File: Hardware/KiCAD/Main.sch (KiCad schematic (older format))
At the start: 33 parts, among them J1 ICSP, J2 DB9, J3 DB9, J4 SPARE, U1 PIC18F25K80, U2 POXA1328-007, U3 RN4020, U4 S25FL127S_SOIC, U5 4000series-4052, U6 4000series-4052, U7 MCP795XX, U8 MAX3232_BJH, U9 MAX3232_BJH, Y1 12MHz, Y2 32.768Hz

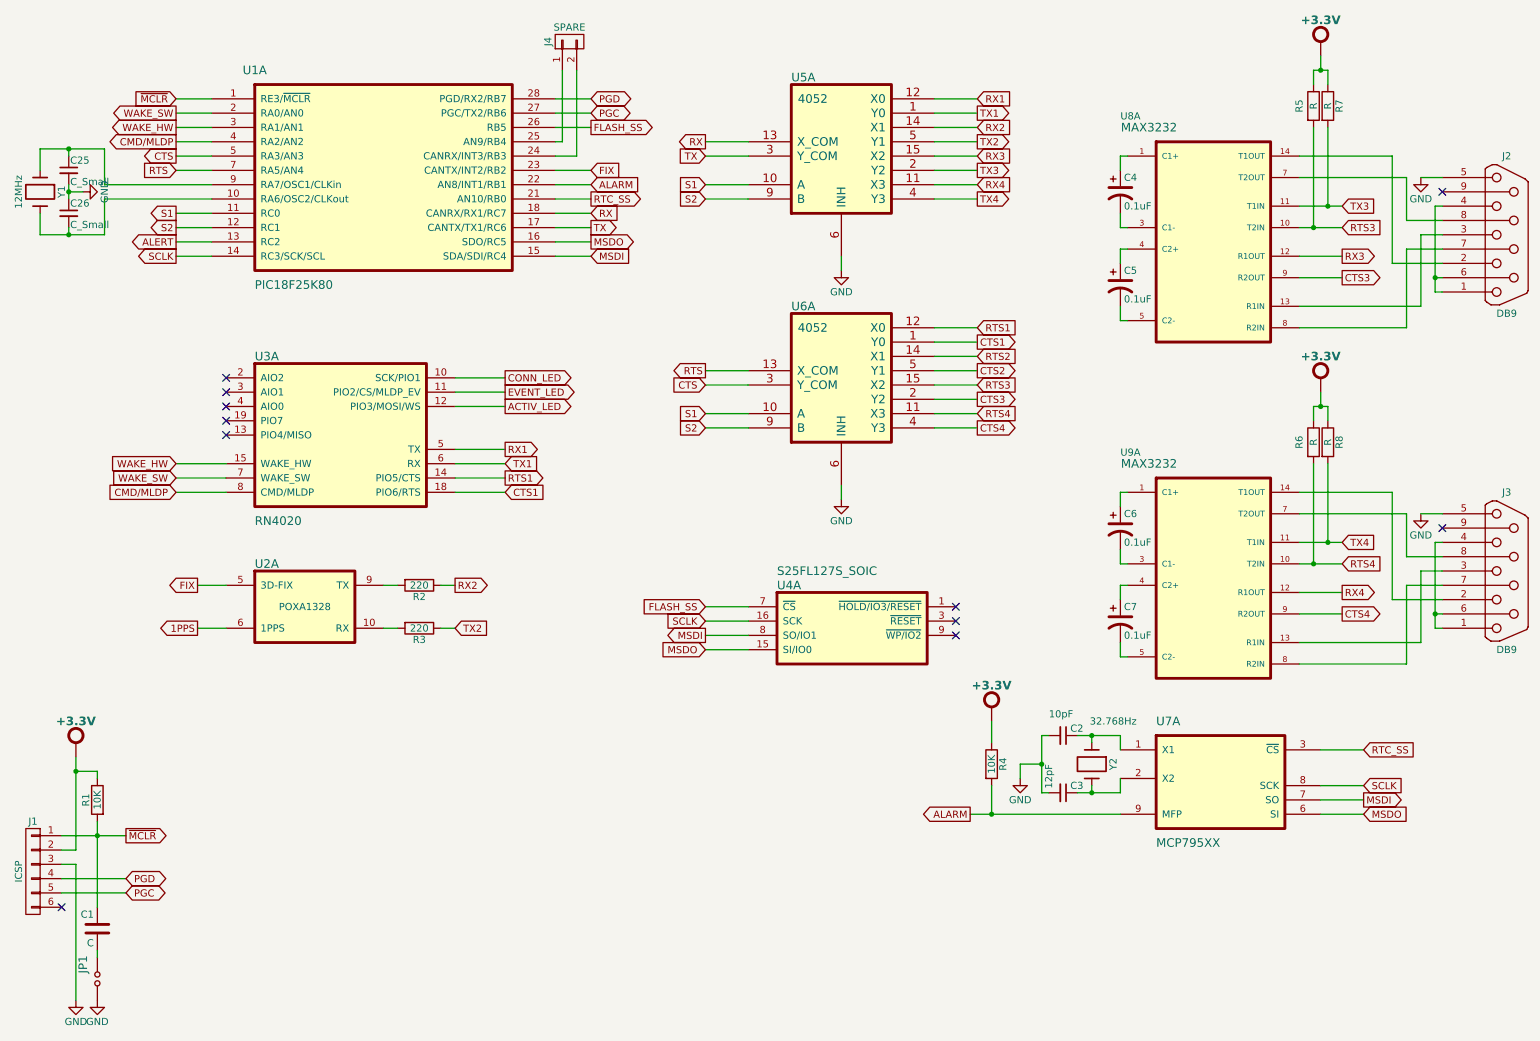
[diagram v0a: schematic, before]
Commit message: More work on PTWS schematic
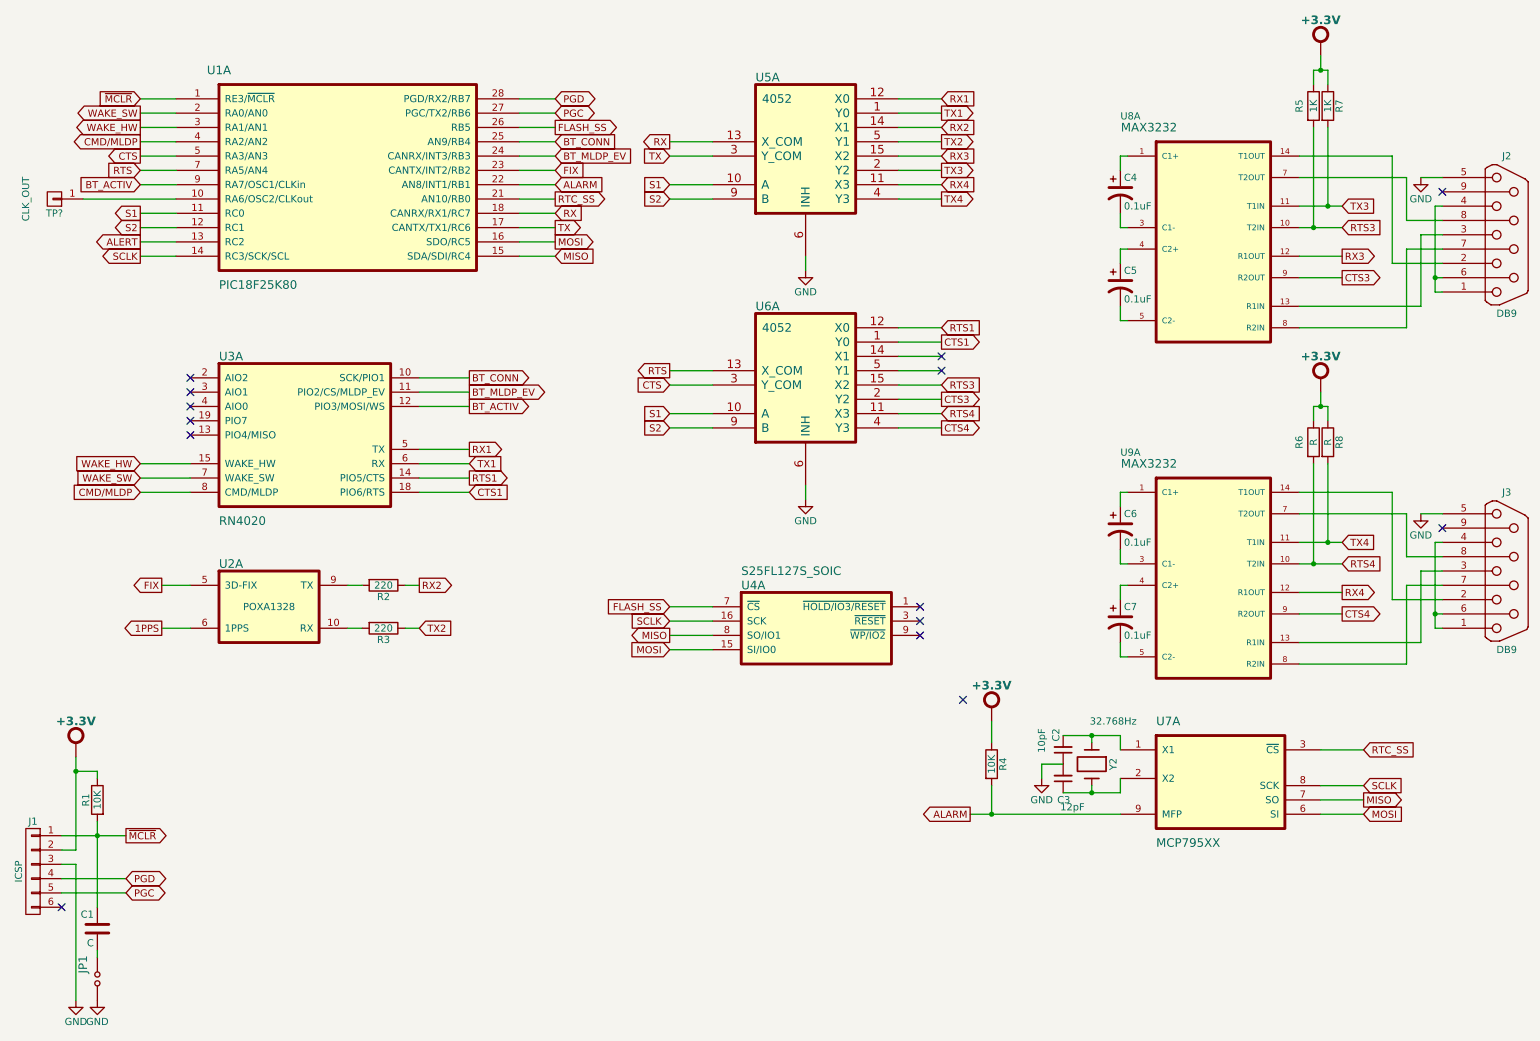
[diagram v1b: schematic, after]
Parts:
- removed C25, C26: C_Small, symbol C_Small
- removed J4: SPARE, symbol CONN_01X02
- removed Y1: 12MHz, symbol Crystal
- added TP?: CLK_OUT, symbol CONN_01X01
- R5, R7: value R -> 1K
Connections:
- net ACTIV_LED is gone; now on net BT_ACTIV: U3.12 (PIO3/MOSI/WS)
- net CONN_LED is gone; now on net BT_CONN: U3.10 (SCK/PIO1)
- net EVENT_LED is gone; now on net BT_MLDP_EV: U3.11 (PIO2/CS/MLDP_EV)
- net GND: now also C2.1; no longer C2.2
- net at U1.10 (RA6/OSC2/CLKout): now also TP?.1 (P1)
- net BT_MLDP_EV: now reaches U1.24 (CANRX/INT3/RB3)
- net BT_CONN: now reaches U1.25 (AN9/RB4)
- net BT_ACTIV: now reaches U1.9 (RA7/OSC1/CLKin)
- net at U7.1 (X1), Y2.1: now also C2.2; no longer C2.1
- net CTS2: no longer names the net of U6.5 (Y1)
- net MSDI renamed MISO
- net MSDO renamed MOSI
- net RTS2: no longer names the net of U6.14 (X1)
- no-connect marks 11 -> 14
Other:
- moved on the sheet: C2, C3, R2, R3, U1A, U2A, U3A, U4A, U5A, U6A

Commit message: more work on the schematic
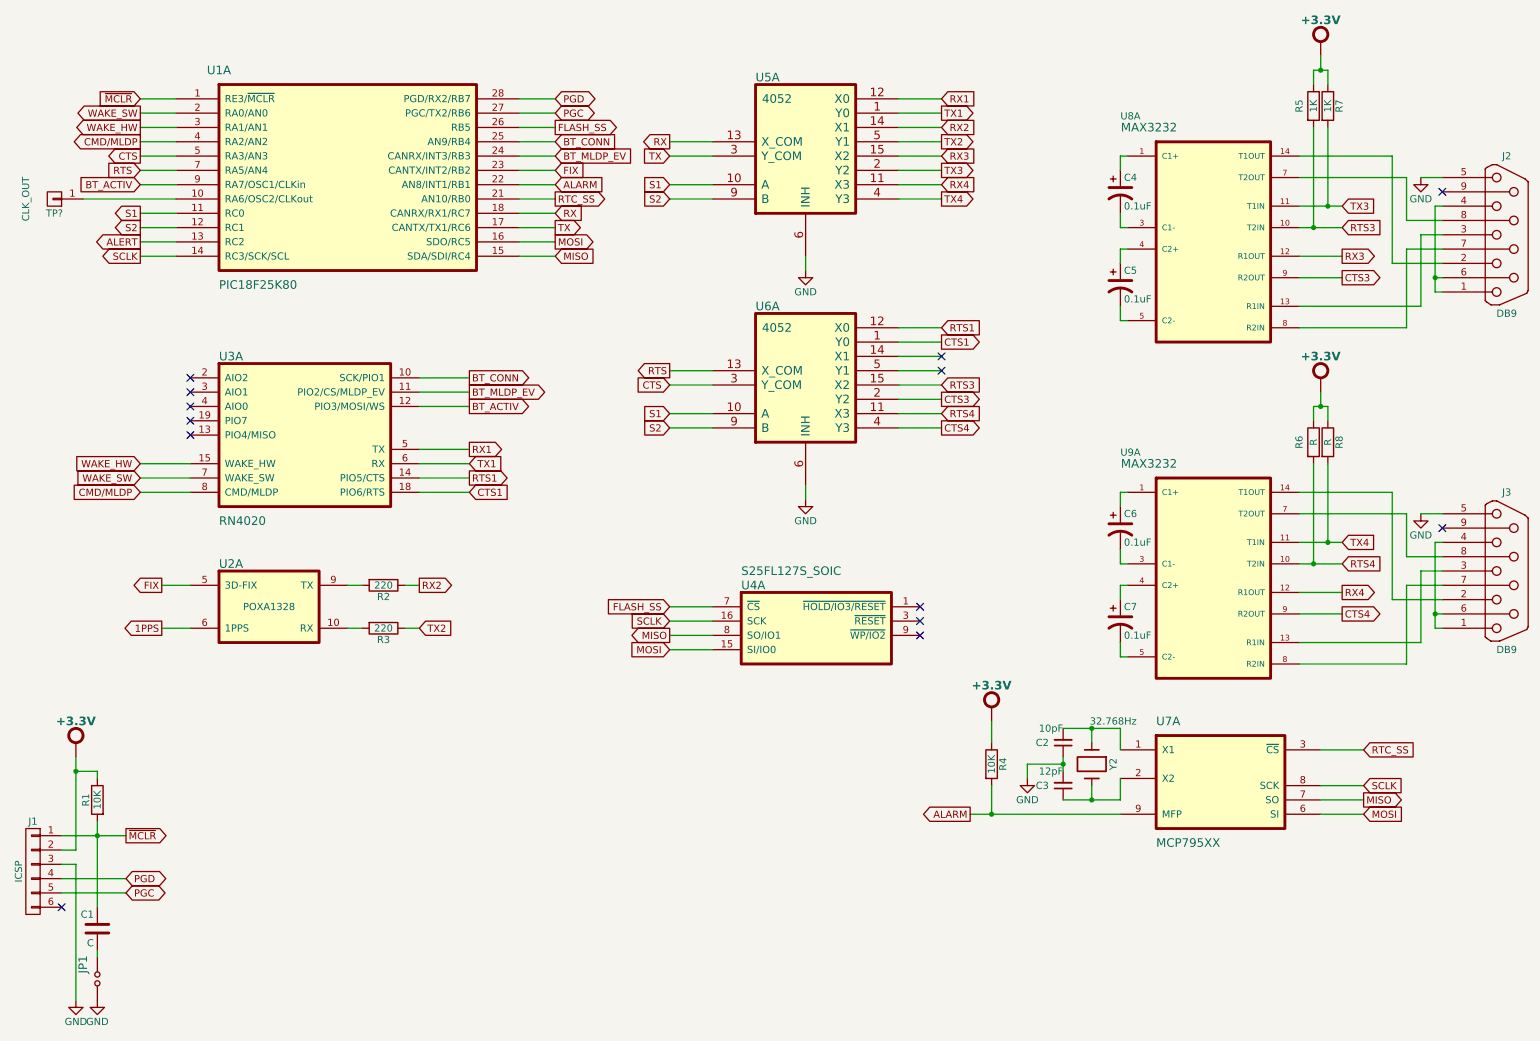
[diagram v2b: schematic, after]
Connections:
- no-connect marks 14 -> 13
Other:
- moved on the sheet: C2, C3
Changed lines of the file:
@@
 LIBS:Relays
 LIBS:Transistors-BJH
+LIBS:MemoryDevices-BJH
 LIBS:ptws-cache
 EELAYER 25 0
@@
 L C_Small C3
 U 1 1 57B87644
-P 7850 5950
-F 0 "C3" H 7800 6100 50  0000 L CNN
-F 1 "12pF" H 7700 6150 50  0000 L CNN
-F 2 "" H 7850 5950 50  0000 C CNN
-F 3 "" H 7850 5950 50  0000 C CNN
-	1    7850 5950
-	-1   0    0    1
-$EndComp
-$Comp
-L C_Small C2
-U 1 1 57B87717
-P 7850 5750
-F 0 "C2" V 7900 5600 50  0000 L CNN
-F 1 "10pF" V 8000 5600 50  0000 L CNN
-F 2 "" H 7850 5750 50  0000 C CNN
-F 3 "" H 7850 5750 50  0000 C CNN
-	1    7850 5750
+P 7850 6000
+F 0 "C3" H 7950 6000 50  0000 L CNN
+F 1 "12pF" H 7850 5900 50  0000 L CNN
+F 2 "" H 7850 6000 50  0000 C CNN
+F 3 "" H 7850 6000 50  0000 C CNN
+	1    7850 6000
 	-1   0    0    1
 $EndComp
@@
 L GND #PWR012
 U 1 1 58010C74
-P 7700 5950
-F 0 "#PWR012" H 7700 5700 50  0001 C CNN
-F 1 "GND" H 7700 5800 50  0000 C CNN
-F 2 "" H 7700 5950 50  0000 C CNN
-F 3 "" H 7700 5950 50  0000 C CNN
-	1    7700 5950
+P 7600 5950
+F 0 "#PWR012" H 7600 5700 50  0001 C CNN
+F 1 "GND" H 7600 5800 50  0000 C CNN
+F 2 "" H 7600 5950 50  0000 C CNN
+F 3 "" H 7600 5950 50  0000 C CNN
+	1    7600 5950
 	1    0    0    -1
 $EndComp
@@
 	9700 1400 9700 1950
 Wire Wire Line
-	9500 1950 9800 1950
-Wire Wire Line
-	9500 2100 9800 2100
+	9500 1950 9700 1950
+Wire Wire Line
+	9700 1950 9800 1950
+Wire Wire Line
+	9500 2100 9600 2100
+Wire Wire Line
+	9600 2100 9800 2100
 Wire Wire Line
 	10250 2050 10500 2050
@@
 	10450 1950 10500 1950
 Wire Wire Line
-	10450 1950 10450 2550
+	10450 1950 10450 2450
+Wire Wire Line
+	10450 2450 10450 2550
 Wire Wire Line
 	10450 2550 10500 2550
@@
 Connection ~ 1100 6350
 Wire Wire Line
-	1100 6250 1100 6850
+	1100 6250 1100 6350
+Wire Wire Line
+	1100 6350 1100 6850
 Connection ~ 950  5900
 Wire Wire Line
@@
 	950  6450 850  6450
 Wire Wire Line
-	950  5800 950  6450
+	950  5800 950  5900
+Wire Wire Line
+	950  5900 950  6450
 Wire Wire Line
 	1300 6750 850  6750
@@
 	1300 6650 850  6650
 Wire Wire Line
-	850  6350 1300 6350
+	850  6350 1100 6350
+Wire Wire Line
+	1100 6350 1300 6350
 Wire Wire Line
 	3350 3350 3700 3350
@@
 	9600 1100 9600 1000
 Wire Wire Line
-	9600 1000 9700 1000
+	9600 1000 9650 1000
+Wire Wire Line
+	9650 1000 9700 1000
 Wire Wire Line
 	9700 1000 9700 1100
@@
 	9700 3750 9700 4300
 Wire Wire Line
-	9500 4300 9800 4300
-Wire Wire Line
-	9500 4450 9800 4450
+	9500 4300 9700 4300
+Wire Wire Line
+	9700 4300 9800 4300
+Wire Wire Line
+	9500 4450 9600 4450
+Wire Wire Line
+	9600 4450 9800 4450
 Wire Wire Line
 	10250 4400 10500 4400
@@
 	10450 4300 10500 4300
 Wire Wire Line
-	10450 4300 10450 4900
+	10450 4300 10450 4800
+Wire Wire Line
+	10450 4800 10450 4900
 Wire Wire Line
 	10450 4900 10500 4900
@@
 	9600 3450 9600 3350
 Wire Wire Line
-	9600 3350 9700 3350
+	9600 3350 9650 3350
+Wire Wire Line
+	9650 3350 9700 3350
 Wire Wire Line
 	9700 3350 9700 3450
@@
 	9950 5750 9650 5750
 Wire Wire Line
-	7200 6200 8250 6200
+	7200 6200 7350 6200
+Wire Wire Line
+	7350 6200 8250 6200
 Wire Wire Line
 	9950 6000 9650 6000
@@
 	9950 6200 9650 6200
 Wire Wire Line
-	8050 5700 8050 5650
-Wire Wire Line
-	8250 5650 8250 5750
-Wire Wire Line
-	8050 6000 8050 6050
-Wire Wire Line
-	8250 6050 8250 5950
-Connection ~ 8050 5650
-Connection ~ 8050 6050
+	8050 5700 8050 5600
+Wire Wire Line
+	8250 5600 8250 5750
+Wire Wire Line
+	8050 6000 8050 6100
+Wire Wire Line
+	8250 6100 8250 5950
+Connection ~ 8050 5600
+Connection ~ 8050 6100
 Wire Wire Line
 	4300 1800 4050 1800
@@
 	4300 1700 4050 1700
 Wire Wire Line
-	7700 5950 7700 5850
+	7600 5950 7600 5850
 Wire Wire Line
 	4050 1600 4300 1600
 Wire Wire Line
-	7850 5650 8250 5650
-Wire Wire Line
-	7850 6050 8250 6050
-Wire Wire Line
-	7700 5850 7850 5850
+	7850 5600 8050 5600
+Wire Wire Line
+	8050 5600 8250 5600
+Wire Wire Line
+	7850 6100 8050 6100
+Wire Wire Line
+	8050 6100 8250 6100
 Text GLabel 4300 1600 2    50   Input ~ 0
 BT_MLDP_EV
@@
 NoConn ~ 7000 3000
 NoConn ~ 7000 3100
-NoConn ~ 7150 5400
+$Comp
+L C_Small C2
+U 1 1 57B87717
+P 7850 5700
+F 0 "C2" H 7950 5700 50  0000 L CNN
+F 1 "10pF" H 7850 5600 50  0000 L CNN
+F 2 "" H 7850 5700 50  0000 C CNN
+F 3 "" H 7850 5700 50  0000 C CNN
+	1    7850 5700
+	-1   0    0    1
+$EndComp
+Wire Wire Line
+	7850 5800 7850 5850
+Wire Wire Line
+	7850 5850 7850 5900
+Wire Wire Line
+	7600 5850 7850 5850
+Connection ~ 7850 5850
 $EndSCHEMATC
